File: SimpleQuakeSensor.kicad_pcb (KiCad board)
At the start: 2 copper layers, 39.9 x 22 mm, 37 parts, among them J1 Conn_Coaxial_Small, J2 Conn_Coaxial_Small, J3 Bat -12V GND, J4 Bat +12V, Q1 2N4401, Q2 BF245B, Q3 2N4401

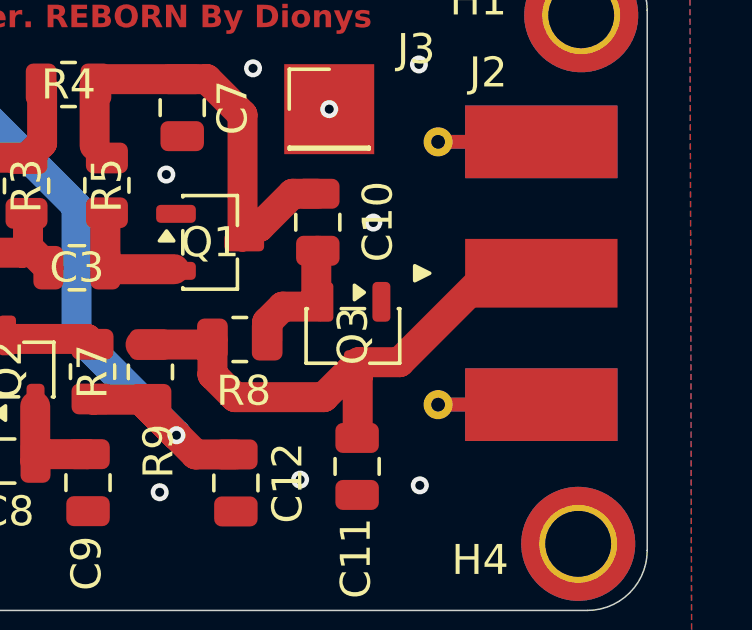
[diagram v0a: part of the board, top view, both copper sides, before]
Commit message: Add blocking capacitor
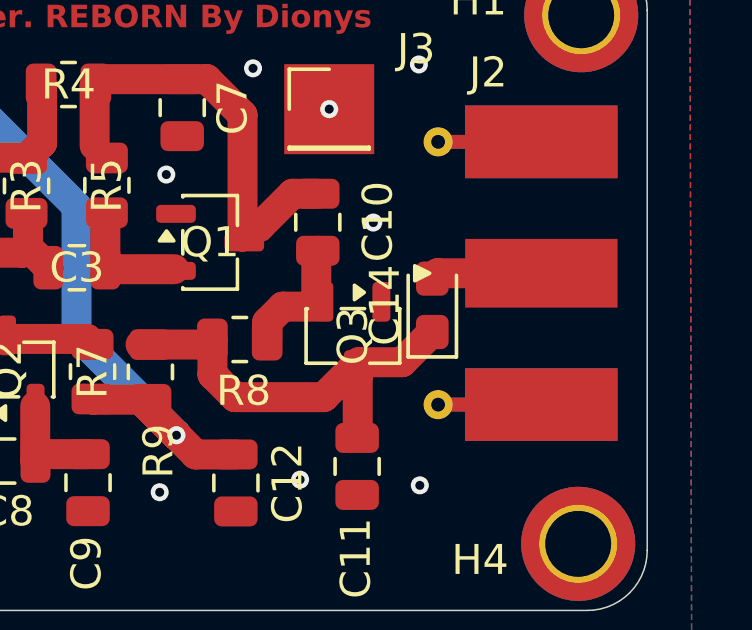
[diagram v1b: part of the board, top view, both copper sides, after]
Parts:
- added C14: 10 uF, Capacitor_Tantalum_SMD:CP_EIA-2012-12_Kemet-R, F.Cu at (166.1, 91.7)
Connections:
- C11 pad 1: Net-(J2-In) -> Net-(Q3-C)
- Q3 pad 3: Net-(J2-In) -> Net-(Q3-C)
- R8 pad 1: Net-(J2-In) -> Net-(Q3-C)
- R9 pad 2: Net-(J2-In) -> Net-(Q3-C)
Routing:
- net Net-(J2-In): track 18.6 -> 3.71 mm
- net Net-(Q3-C): track 0.00 -> 14.2 mm
